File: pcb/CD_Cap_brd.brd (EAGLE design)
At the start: 149.9 x 45.7 mm, 18 parts, among them Q1 IRF3704S, Q2 IRF3704S

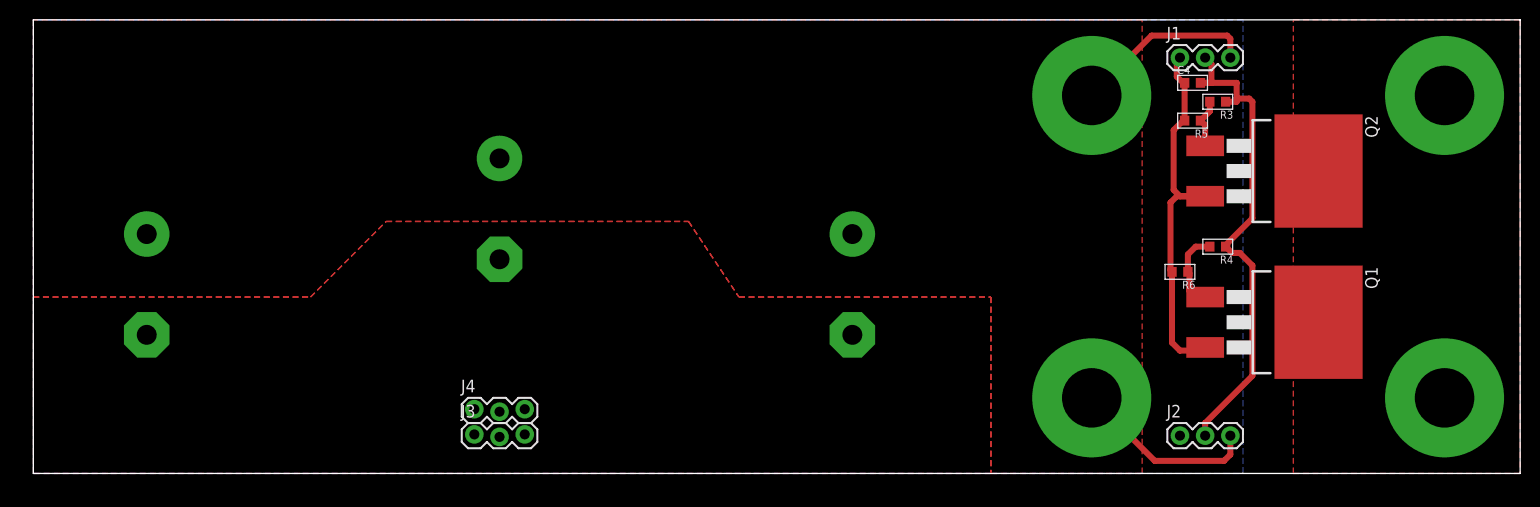
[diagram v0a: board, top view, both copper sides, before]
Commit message: almost ready for FAB
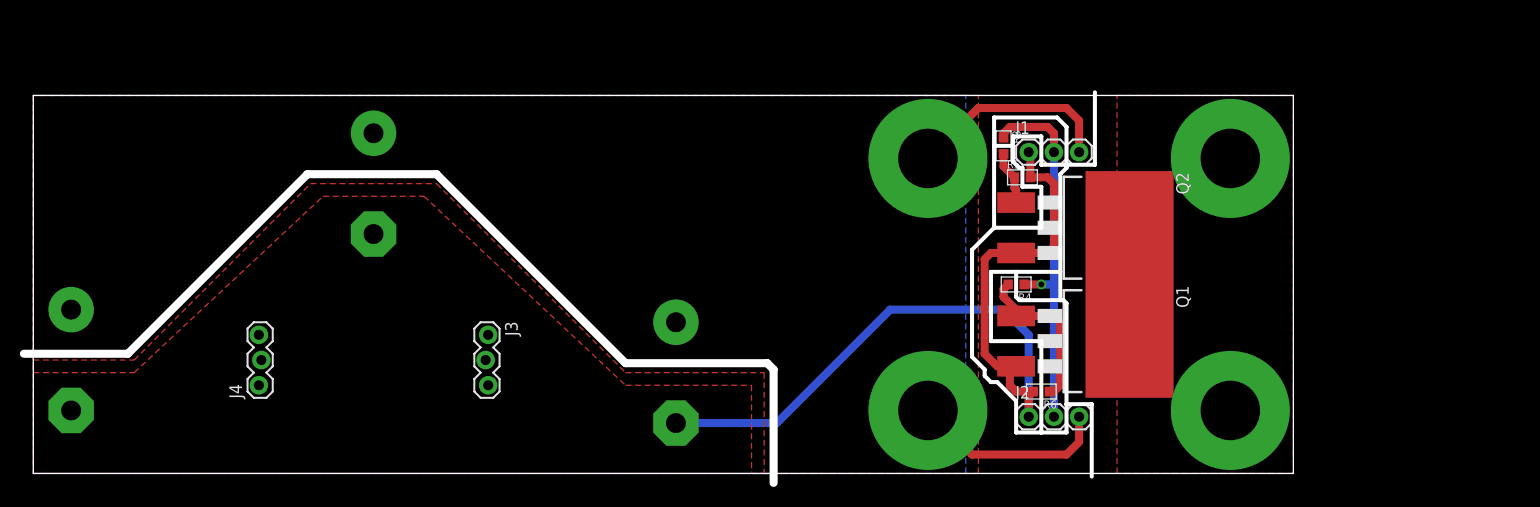
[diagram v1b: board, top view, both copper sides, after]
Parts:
- removed C4: (no value), passives-7351:C0603-N
- moved U$3 22.5 mm to (120.7, 31.8)
- moved R3 22.0 mm to (97.8, 33.0), turned to 270 degrees
- moved J4 21.7 mm to (22.9, 8.89), turned to 90 degrees
- moved U$4 21.6 mm to (120.7, 6.35)
- moved R4 20.7 mm to (99.1, 19.1)
- moved Q2 19.9 mm to (108.0, 24.8)
- moved C8 19.9 mm to (64.8, 10.2)
- moved Q1 19.1 mm to (108.0, 13.3)
- moved R6 18.5 mm to (101.6, 8.26)
- moved R5 18.1 mm to (99.7, 29.8), turned to 0 degrees
- moved J1 18.0 mm to (100.3, 32.4)
- moved U$1 17.7 mm to (90.2, 31.8)
- moved U$2 16.6 mm to (90.2, 6.35)
- moved J2 15.4 mm to (100.3, 5.71)
- moved C7 13.0 mm to (34.3, 29.2)
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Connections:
- net B-: no longer C4.1
- net TRIG: no longer C4.2
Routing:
- net B-: track 39.6 -> 89.5 mm
- net TRIG: track 49.5 -> 37.7 mm, vias 0 -> 1
- net N$1: track 8.11 -> 16.3 mm
- net B+: track 37.3 -> 41.2 mm
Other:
- board size 149.9 x 45.7 mm -> 128 x 39.4 mm
